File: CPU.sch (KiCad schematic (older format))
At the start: 131 parts, among them J1 Conn_01x30, J2 Conn_01x30, J3 Conn_01x24, SW1 SW_Push, SW2 SW_Push, SW3 SW_Push, SW4 SW_Push, U1 USB_MICRO, U10 GD5F1GQ4UAYIG, U11 EA3036, U12 XC6206, U13 HR911105A, U2 NS2009, U3 FC-40P-LCD, U4 allwinner-V3S-eLQFP128, U5 TF_CARD, U6 MC-146, U7 MX25L12835F, U8 PT4101, U9 XT_3225

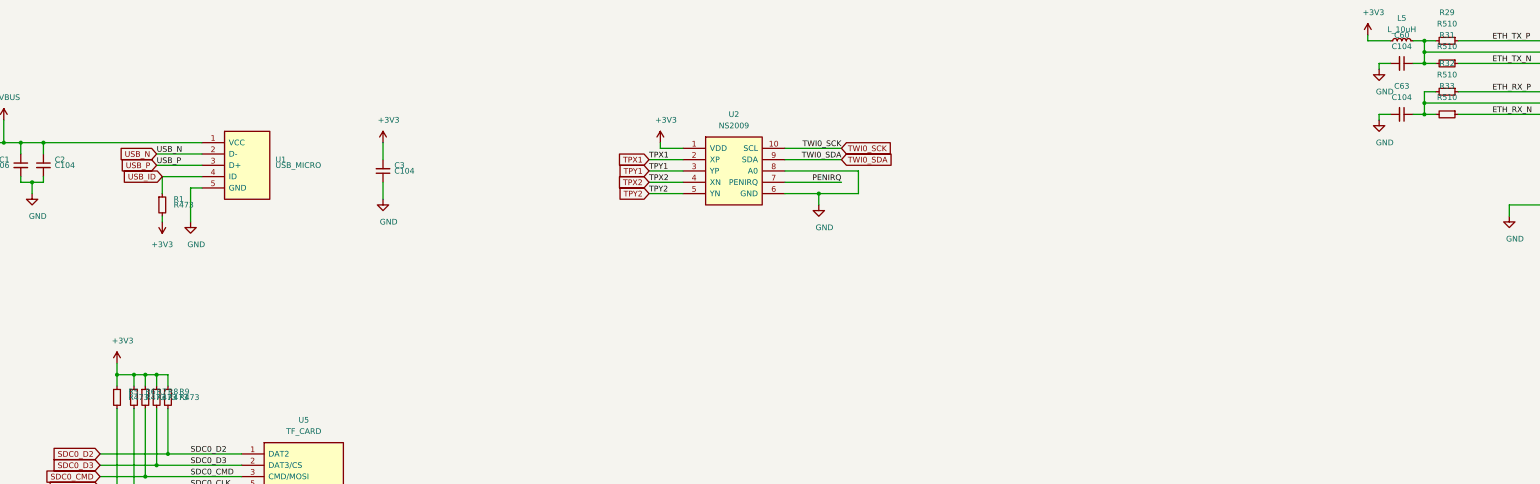
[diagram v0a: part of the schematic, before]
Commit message: update,
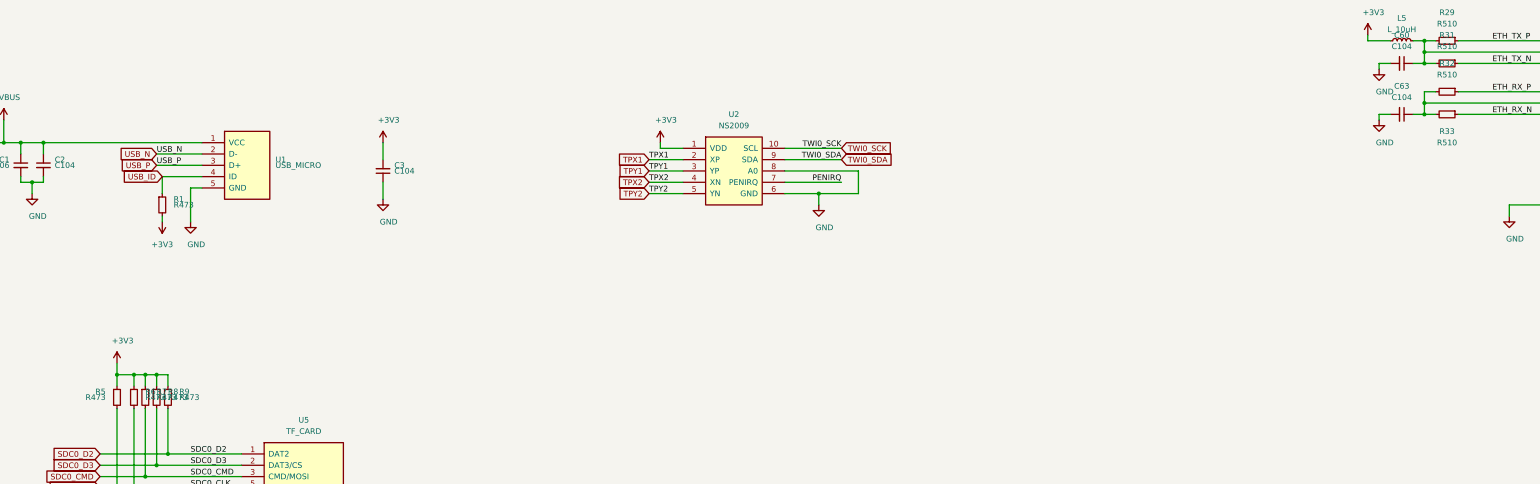
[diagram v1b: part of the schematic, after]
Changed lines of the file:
@@
 AR Path="/5BCCA602/5BFB14AD" Ref="R?"  Part="1"
 AR Path="/5BCC9E7B/5BFB14AD" Ref="R5"  Part="1"
-F 0 "R5" H 22300 4700 50  0000 L CNN
-F 1 "R473" H 22300 4650 50  0000 L CNN
+F 0 "R5" H 22100 4700 50  0000 R CNN
+F 1 "R473" H 22100 4650 50  0000 R CNN
 F 2 "Resistor_SMD:R_0603_1608Metric_Pad1.05x0.95mm_HandSolder" H 22200 4650 50  0001 C CNN
 F 3 "~" H 22200 4650 50  0001 C CNN
@@
 U 1 1 5C4CCCAA
 P 33950 2150
-F 0 "R33" V 33700 2150 50  0000 C CNN
-F 1 "R510" V 33800 2150 50  0000 C CNN
+F 0 "R33" V 34100 2150 50  0000 C CNN
+F 1 "R510" V 34200 2150 50  0000 C CNN
 F 2 "Resistor_SMD:R_0603_1608Metric_Pad1.05x0.95mm_HandSolder" H 33950 2150 50  0001 C CNN
 F 3 "~" H 33950 2150 50  0001 C CNN
